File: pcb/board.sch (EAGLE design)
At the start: 21 parts, among them Q1 MPSA42

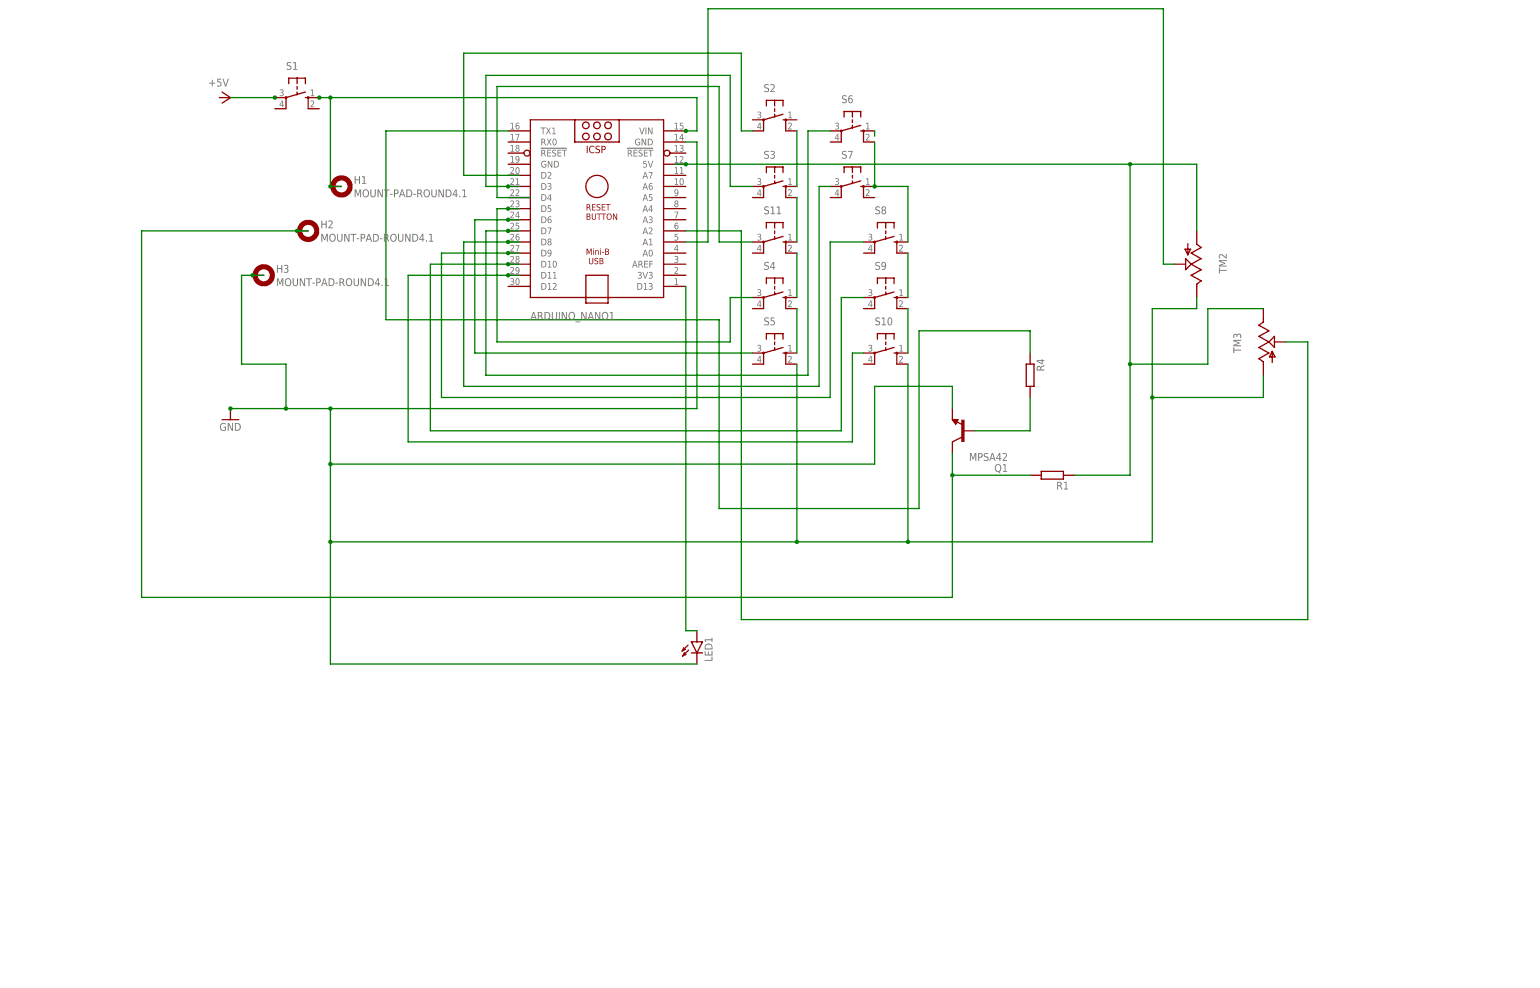
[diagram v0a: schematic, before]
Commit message: Clean-up repository
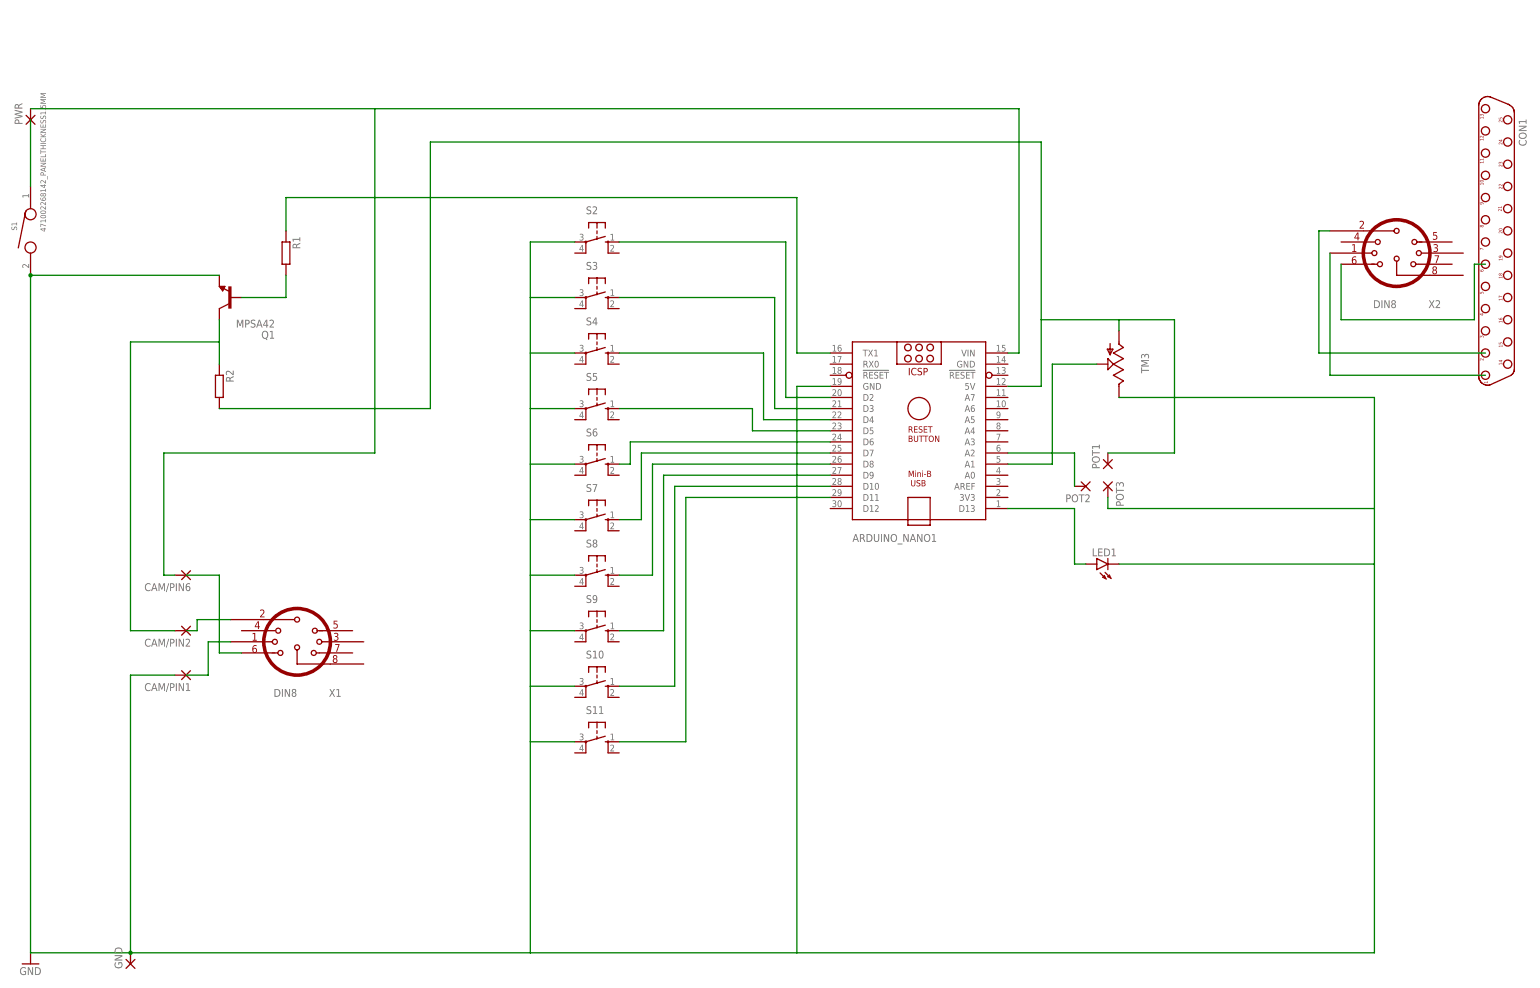
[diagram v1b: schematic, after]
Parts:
- removed H1, H2, H3: MOUNT-PAD-ROUND4.1, holes:MOUNT-PAD-ROUND4.1
- removed R4: (no value), rcl:R-EU_0204/2V
- removed TM2: (no value), Bourns PTA series:TRIMSLIDE75
- added CAM/PIN1, CAM/PIN2, CAM/PIN6, GND, POT1, POT2, POT3, PWR: (no value), wirepad:1,6/0,8
- added CON1: (no value), db25:DB25F
- added R2: (no value), rcl:R-EU_0204/2V
- added X1, X2: DIN8, con-din8:DIN8
- S1: value (none) -> 471002268142_PANELTHICKNESS1.5MM; device switch-omron:40-XX -> power_switch:471002268142_PANELTHICKNESS1.5MM
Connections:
- removed net N$19 (its old number): ARDUINO_NANO1.A2, TM3.WIPER
- removed net N$26: S10.S, S9.S1
- removed net N$27: S11.S1, S4.S
- new net GND: ARDUINO_NANO1.GND@1, CAM/PIN1.P, GND.P, LED1.C, POT3.P, Q1.E, S1.2, S10.P, S11.P, S2.P, S3.P, S4.P, S5.P, S6.P, S7.P, S8.P, S9.P, TM3.B
- net N$1: now also X1.7; no longer S1.P
- net N$10: now also S9.S; no longer S8.P
- net N$11: now also S10.S; no longer S9.P
- net N$12: now also S11.S; no longer S10.P
- net N$13: now also ARDUINO_NANO1.VIN, CAM/PIN6.P, PWR.P; no longer ARDUINO_NANO1.D2, S2.P1
- net N$14: now also ARDUINO_NANO1.TX1, R1.1; no longer ARDUINO_NANO1.D4, S11.P
- net N$15: now also Q1.B, R1.2; no longer ARDUINO_NANO1.TX1, R4.1
- net N$16: now also ARDUINO_NANO1.A1, TM3.WIPER; no longer H2.MOUNT, Q1.C, R1.2
- net N$17: now also ARDUINO_NANO1.A2, POT2.P; no longer ARDUINO_NANO1.5V, R1.1, TM2.A, TM3.B
- net N$18: now also CAM/PIN2.P, Q1.C, R2.1; no longer ARDUINO_NANO1.A1, TM2.WIPER
- net N$2: now also ARDUINO_NANO1.5V, POT1.P, R2.2, TM3.A; no longer ARDUINO_NANO1.VIN, H1.MOUNT, S1.S
- net N$20: now also X1.2; no longer S2.S1, S3.S
- net N$21: now also X1.1; no longer S11.S, S3.S1
- net N$22: now also CON1.2, X2.2; no longer S4.S1, S5.S
- net N$23: now also CON1.6, X2.7; no longer S6.S
- net N$24: now also CON1.1, X2.1; no longer S6.S1, S7.S, S8.S
- net N$25: now also S1.1; no longer S8.S1, S9.S
- net N$3: now also ARDUINO_NANO1.D2, S2.S; no longer ARDUINO_NANO1.GND@2, H3.MOUNT, LED1.C, Q1.E, S10.S1, S5.S1, TM2.B, TM3.A
- net N$4: now also ARDUINO_NANO1.D3, S3.S; no longer Q1.B, R4.2
- net N$5: now also ARDUINO_NANO1.D4, S4.S; no longer ARDUINO_NANO1.D3, S3.P
- net N$6: now also ARDUINO_NANO1.D5, S5.S; no longer ARDUINO_NANO1.D7, S6.P
- net N$7: now also ARDUINO_NANO1.D6, S6.S; no longer ARDUINO_NANO1.D5, S4.P
- net N$8: now also ARDUINO_NANO1.D7, S7.S; no longer ARDUINO_NANO1.D6, S5.P
- net N$9: now also S8.S; no longer S7.P
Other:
- moved on the sheet: ARDUINO_NANO1, LED1, Q1, R1, S10, S11, S2, S3, S4, S5, S6, S7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
